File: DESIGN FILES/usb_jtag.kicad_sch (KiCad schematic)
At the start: 10 parts

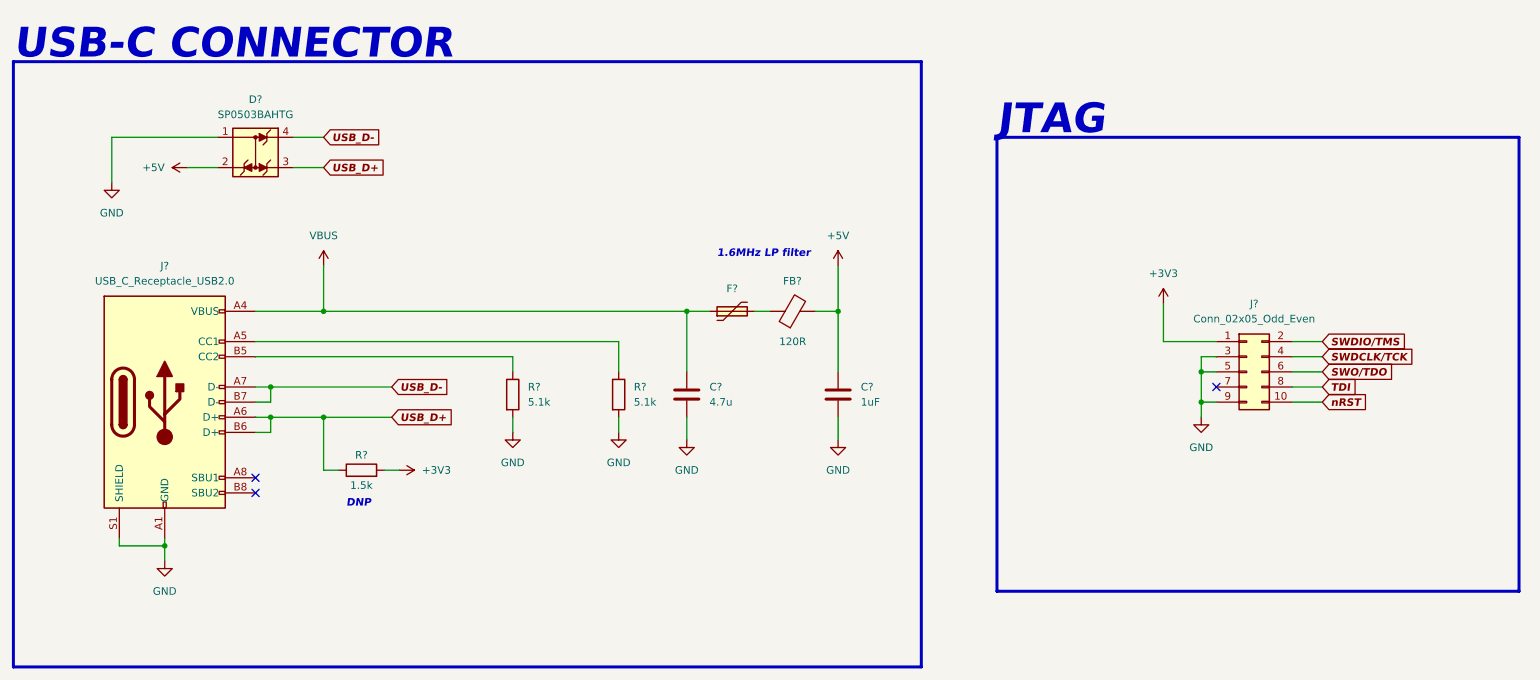
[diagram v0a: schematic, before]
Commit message: updates
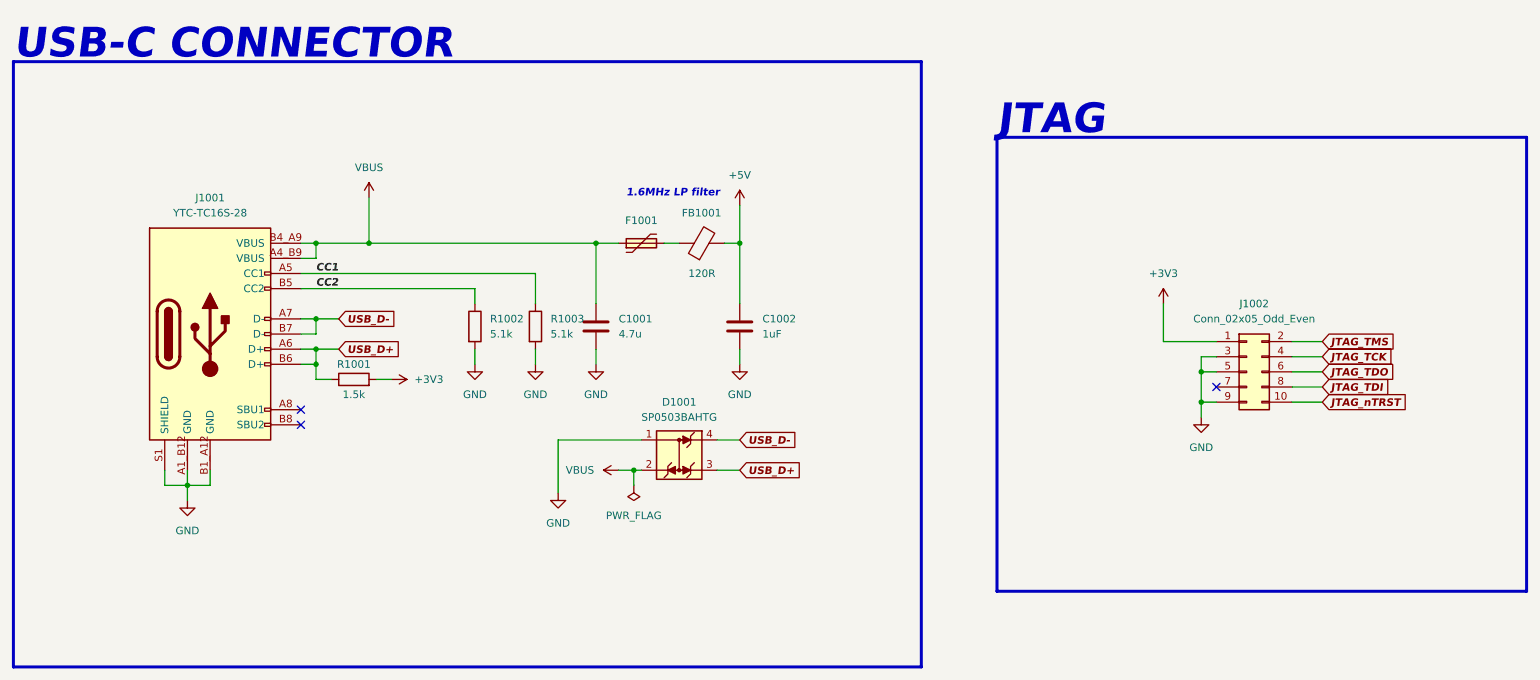
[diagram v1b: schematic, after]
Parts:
- removed C?: 1uF, symbol MY CAPACITOR LIBRARY:CL10A105KB8NNNC
- removed C?: 4.7u, symbol MY CAPACITOR LIBRARY:CL10A475KO8NNNC
- removed D?: SP0503BAHTG, digikey-footprints:SOT-143-4, symbol MY DIODE LIBRARY:SP0503BAHTG
- removed F?: SMD0805P020TF, symbol MY FUSE LIBRARY:SMD0805P020TF
- removed FB?: 120R, symbol MY FERRITE BEAD LIBRARY:BLM18AG121SN1D
- removed J?: USB_C_Receptacle_USB2.0, symbol MY CONNECTOR LIBRARY:USB_C_Receptacle_USB2.0
- removed R? (x2): 5.1k, symbol MY RESISTOR LIBRARY:0603WAF5101T5E
- removed R?: 1.5k, symbol MY RESISTOR LIBRARY:CQ03WAJ0152T5E
- added C1001: 4.7u, MY CAPACITOR LIBRARY:CL10A475KO8NNNC_0603, symbol MY CAPACITOR LIBRARY:CL10A475KO8NNNC
- added C1002: 1uF, MY CAPACITOR LIBRARY:CL10A105KB8NNNC_0603, symbol MY CAPACITOR LIBRARY:CL10A105KB8NNNC
- added D1001: SP0503BAHTG, MY DIODE LIBRARY:SP0503BAHTG_SOT-143, symbol MY DIODE LIBRARY:SP0503BAHTG
- added F1001: SMD0805P020TF, MY FUSE LIBRARY:0805_SMD0805P020TF, symbol MY FUSE LIBRARY:SMD0805P020TF
- added FB1001: 120R, MY FERRITE BEAD LIBRARY:0603_BLM18AG121SN1D, symbol MY FERRITE BEAD LIBRARY:BLM18AG121SN1D
- added J1001: YTC-TC16S-28, MY CONNECTOR LIBRARY:YTC-TC16S-28, symbol MY CONNECTOR LIBRARY:YTC-TC16S-28
- added R1001: 1.5k, MY RESISTOR LIBRARY:CQ03WAJ0152T5E, symbol MY RESISTOR LIBRARY:CQ03WAJ0152T5E
- added R1002, R1003: 5.1k, MY RESISTOR LIBRARY:0603WAF5101T5E, symbol MY RESISTOR LIBRARY:0603WAF5101T5E
- J1002: renamed from J?; footprint (none) -> MY CONNECTOR LIBRARY:PZ127VS-12-10-H10-A38
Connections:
- net +3V3: now also R1001.2
- net +5V: now also C1002.1, FB1001.2
- net GND: now also C1001.2, C1002.2, D1001.1, J1001.A1_B12 (GND), J1001.B1_A12 (GND), J1001.S1 (SHIELD), R1002.2, R1003.2
- net USB_D+: now also D1001.3, J1001.A6 (D+), J1001.B6 (D+), R1001.1
- net USB_D-: now also D1001.4, J1001.A7 (D-), J1001.B7 (D-)
- net VBUS: now also C1001.1, D1001.2, F1001.1, J1001.A4_B9 (VBUS), J1001.B4_A9 (VBUS)
- net SWDCLK/TCK renamed JTAG_TCK
- net SWDIO/TMS renamed JTAG_TMS
- net SWO/TDO renamed JTAG_TDO
- net TDI renamed JTAG_TDI
- net nRST renamed JTAG_nTRST
- new net: F1001.2, FB1001.1
- new net CC1: J1001.A5 (CC1), R1003.1
- new net CC2: J1001.B5 (CC2), R1002.1
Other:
- note removed: "DNP"
